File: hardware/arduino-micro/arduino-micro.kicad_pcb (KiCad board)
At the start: 2 copper layers, 76.5 x 46.5 mm, 26 parts, among them J1 PJ-088CH, J2 i2c_header, M1 Fan_4pin, SW1 Rotary_Encoder, U1 TM1637, U2 CA56-12CGKWA, U3 BUTTON_1, U4 BUTTON_2, U5 BUTTON_3

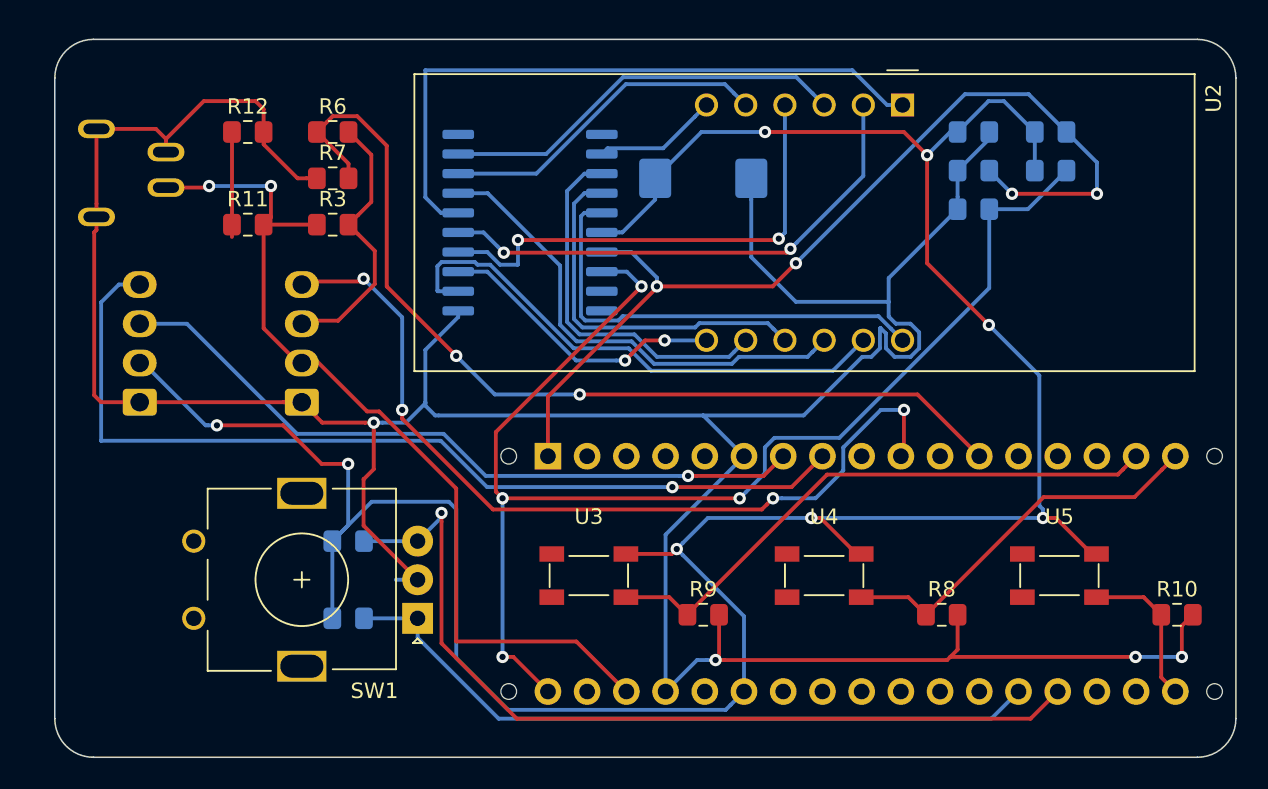
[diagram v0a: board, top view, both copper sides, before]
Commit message: board updates for prototype
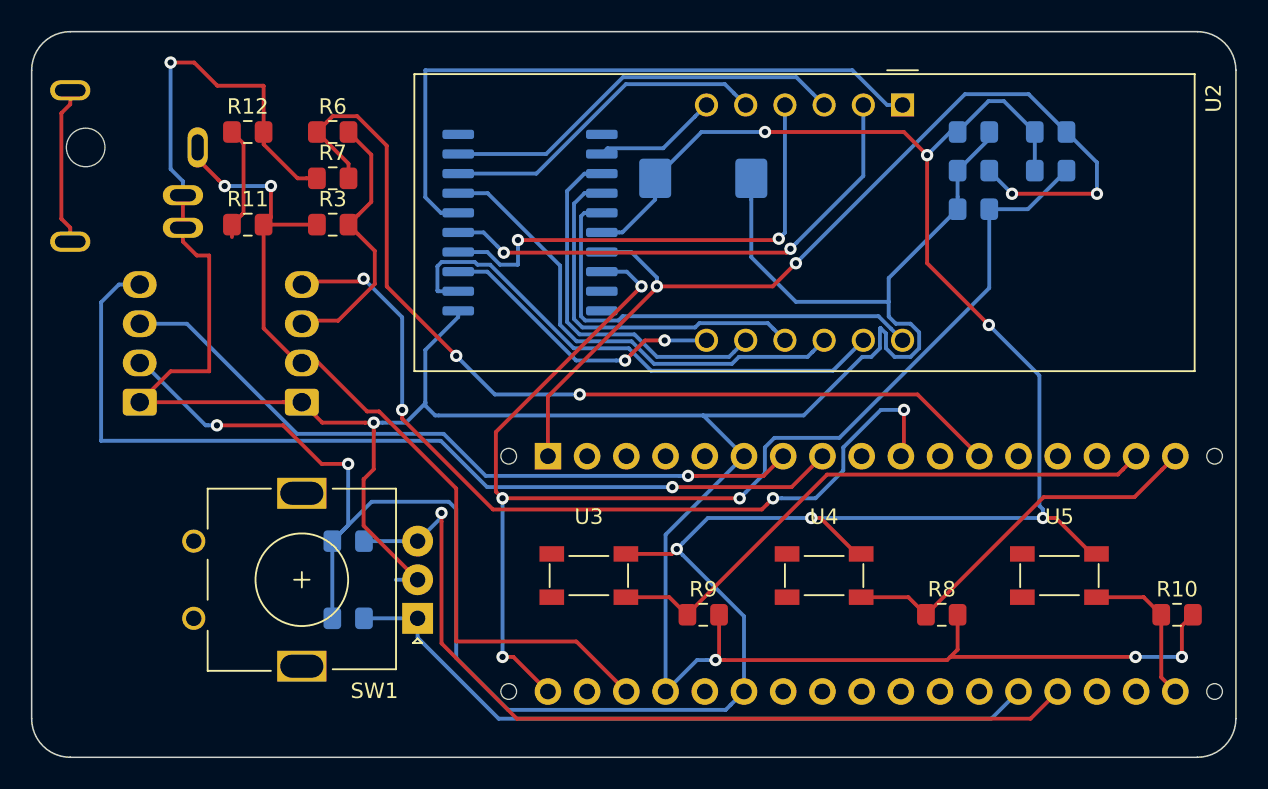
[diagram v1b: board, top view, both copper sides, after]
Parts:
- J1: value PJ-088CH -> PJ-083H; footprint PJ-088CH:CUI_PJ-088CH -> squeeze-misc:CUI_PJ-083H
- moved J1 2.83 mm to (112.0, 98.0)
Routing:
- net Net-(J1-PadS1): track 0.00 -> 10.3 mm
- net GND: track 216.1 -> 217.5 mm, vias 4 -> 5
- net Net-(J2-Pad2): track 6.80 -> 7.42 mm
- net +12V: track 59.8 -> 59.2 mm
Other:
- board size 76.5 x 46.5 mm -> 78 x 47 mm
